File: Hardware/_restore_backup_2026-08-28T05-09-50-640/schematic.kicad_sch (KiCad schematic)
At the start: 6 parts, among them U1 ESP32-WROOM-32E, U2 HX711, U5 MAX30102, U6 MPU-6050

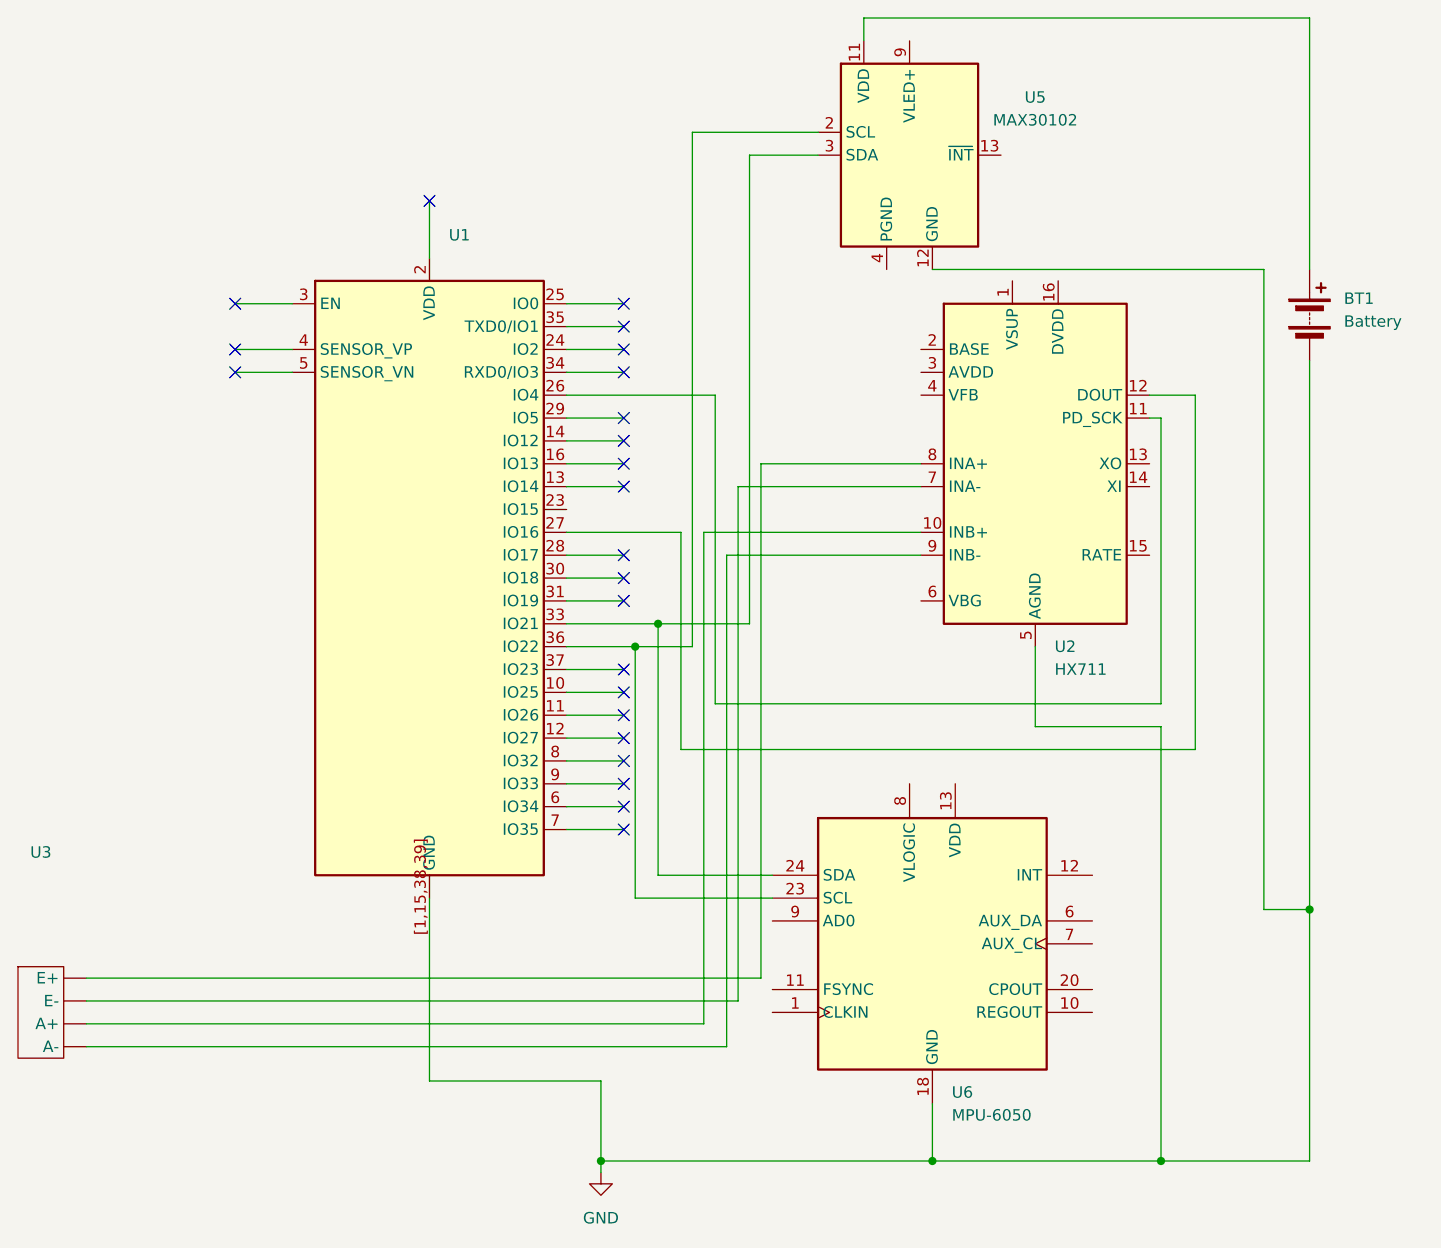
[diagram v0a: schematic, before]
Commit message: feat: added full structure to the project
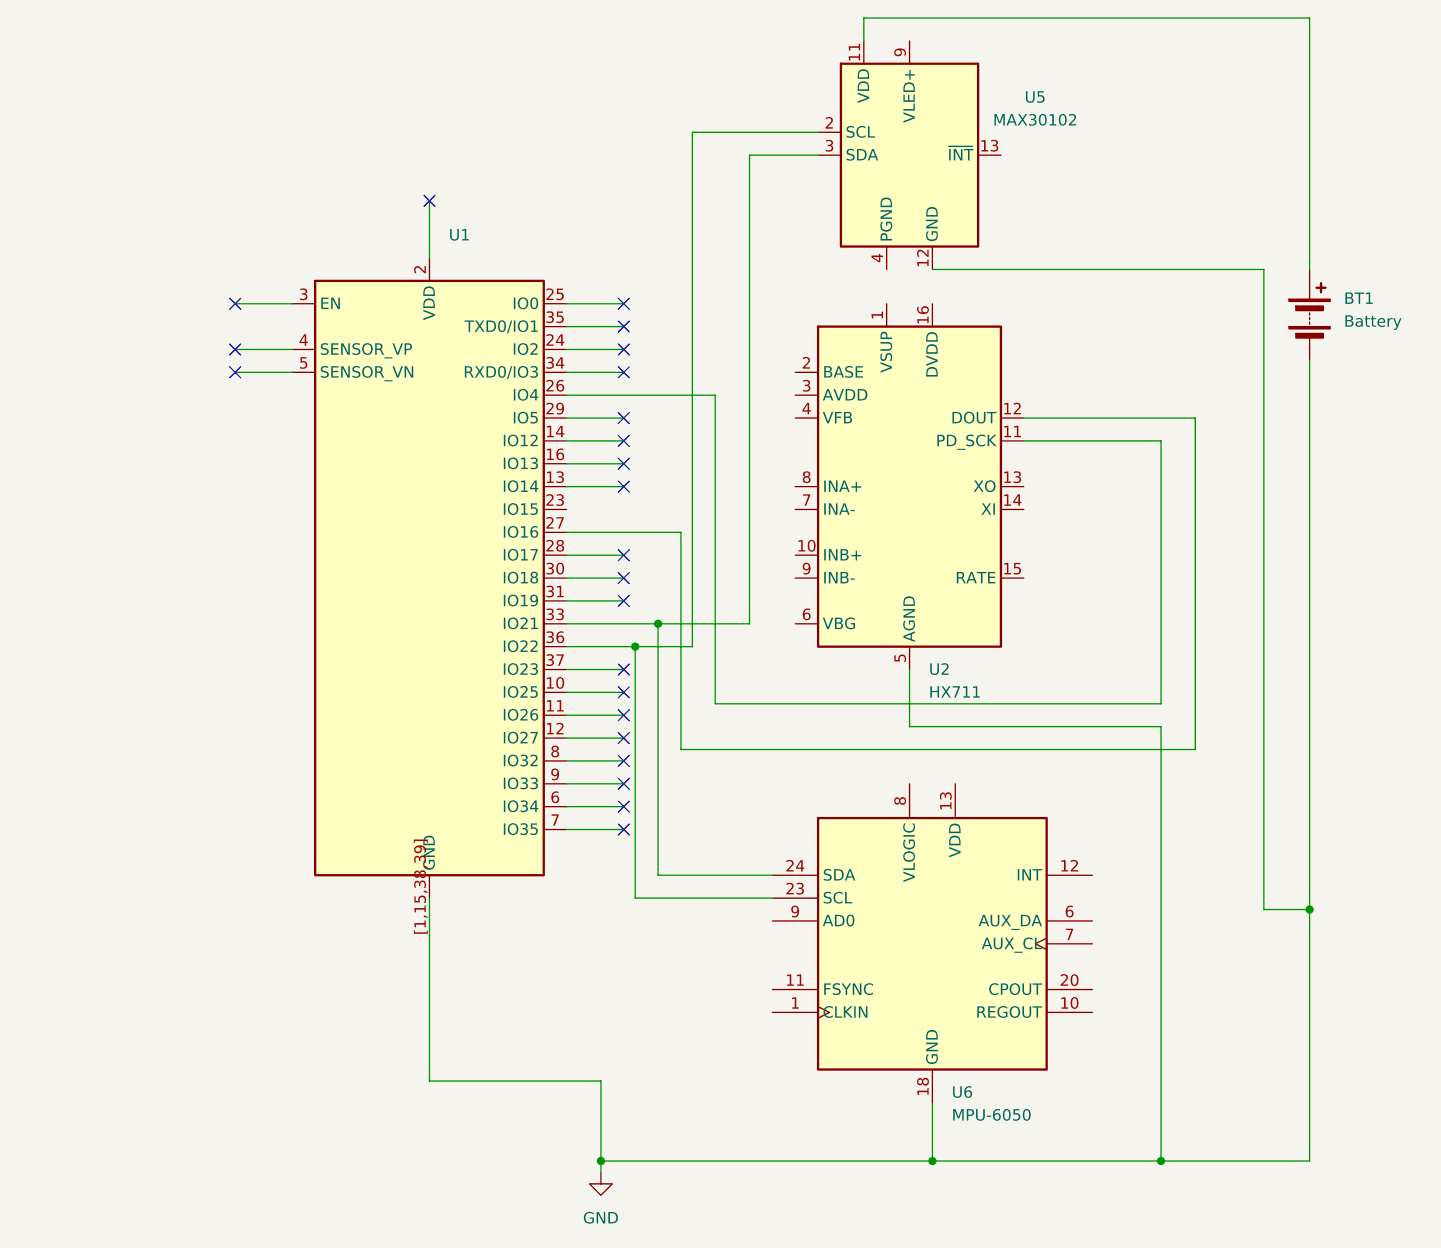
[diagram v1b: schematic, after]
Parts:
- removed U3: (no value), symbol New_Library:LOAD_CELL
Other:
- moved on the sheet: U2
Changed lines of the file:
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@@
-	(wire
-		(pts
-			(xy 179.07 78.74) (xy 196.85 78.74)
-		)
-		(stroke
-			(width 0)
-			(type default)
-		)
-	)
 	(wire
 		(pts
@@
 	(wire
 		(pts
-			(xy 172.72 86.36) (xy 196.85 86.36)
-		)
-		(stroke
-			(width 0)
-			(type default)
-		)
-	)
-	(wire
-		(pts
 			(xy 120.65 68.58) (xy 127 68.58)
 		)
@@
 	(wire
 		(pts
-			(xy 222.25 71.12) (xy 227.33 71.12)
-		)
-		(stroke
-			(width 0)
-			(type default)
-		)
-	)
-	(wire
-		(pts
-			(xy 176.53 138.43) (xy 176.53 81.28)
+			(xy 208.28 73.66) (xy 227.33 73.66)
 		)
 		(stroke
@@
 	(wire
 		(pts
-			(xy 104.14 140.97) (xy 172.72 140.97)
-		)
-		(stroke
-			(width 0)
-			(type default)
-		)
-	)
-	(wire
-		(pts
 			(xy 171.45 41.91) (xy 185.42 41.91)
 		)
@@
 	(wire
 		(pts
-			(xy 209.55 107.95) (xy 209.55 99.06)
+			(xy 195.58 107.95) (xy 195.58 101.6)
 		)
 		(stroke
@@
 	(wire
 		(pts
-			(xy 223.52 107.95) (xy 209.55 107.95)
+			(xy 223.52 107.95) (xy 195.58 107.95)
 		)
 		(stroke
@@
 	(wire
 		(pts
-			(xy 104.14 138.43) (xy 176.53 138.43)
-		)
-		(stroke
-			(width 0)
-			(type default)
-		)
-	)
-	(wire
-		(pts
 			(xy 163.83 101.6) (xy 157.48 101.6)
 		)
@@
 	(wire
 		(pts
-			(xy 172.72 140.97) (xy 172.72 86.36)
-		)
-		(stroke
-			(width 0)
-			(type default)
-		)
-	)
-	(wire
-		(pts
 			(xy 163.83 60.96) (xy 157.48 60.96)
 		)
@@
 	(wire
 		(pts
-			(xy 179.07 135.89) (xy 179.07 78.74)
-		)
-		(stroke
-			(width 0)
-			(type default)
-		)
-	)
-	(wire
-		(pts
 			(xy 142.24 147.32) (xy 161.29 147.32)
 		)
@@
 	(wire
 		(pts
-			(xy 176.53 81.28) (xy 196.85 81.28)
-		)
-		(stroke
-			(width 0)
-			(type default)
-		)
-	)
-	(wire
-		(pts
 			(xy 170.18 86.36) (xy 157.48 86.36)
 		)
@@
 	(wire
 		(pts
-			(xy 104.14 143.51) (xy 175.26 143.51)
-		)
-		(stroke
-			(width 0)
-			(type default)
-		)
-	)
-	(wire
-		(pts
 			(xy 163.83 68.58) (xy 157.48 68.58)
 		)
@@
 	(wire
 		(pts
-			(xy 175.26 88.9) (xy 196.85 88.9)
-		)
-		(stroke
-			(width 0)
-			(type default)
-		)
-	)
-	(wire
-		(pts
-			(xy 227.33 71.12) (xy 227.33 110.49)
-		)
-		(stroke
-			(width 0)
-			(type default)
-		)
-	)
-	(wire
-		(pts
-			(xy 223.52 73.66) (xy 223.52 105.41)
+			(xy 227.33 73.66) (xy 227.33 110.49)
+		)
+		(stroke
+			(width 0)
+			(type default)
+		)
+	)
+	(wire
+		(pts
+			(xy 223.52 76.2) (xy 223.52 105.41)
 		)
 		(stroke
@@
 	(wire
 		(pts
-			(xy 104.14 135.89) (xy 179.07 135.89)
-		)
-		(stroke
-			(width 0)
-			(type default)
-		)
-	)
-	(wire
-		(pts
 			(xy 223.52 105.41) (xy 173.99 105.41)
 		)
@@
 	(wire
 		(pts
-			(xy 175.26 143.51) (xy 175.26 88.9)
-		)
-		(stroke
-			(width 0)
-			(type default)
-		)
-	)
-	(wire
-		(pts
 			(xy 198.12 156.21) (xy 198.12 149.86)
 		)
@@
 	(wire
 		(pts
-			(xy 222.25 73.66) (xy 223.52 73.66)
+			(xy 208.28 76.2) (xy 223.52 76.2)
 		)
 		(stroke
@@
 	)
 	(symbol
-		(lib_id "New_Library:LOAD_CELL")
-		(at 100.33 124.46 0)
-		(unit 1)
-		(body_style 1)
-		(exclude_from_sim no)
-		(in_bom yes)
-		(on_board yes)
-		(in_pos_files yes)
-		(dnp no)
-		(fields_autoplaced yes)
-		(property "Reference" "U3"
-			(at 99.06 121.92 0)
-			(show_name no)
-			(do_not_autoplace no)
-			(effects
-				(font
-					(size 1.27 1.27)
-				)
-			)
-		)
-		(property "Value" ""
-			(at 100.33 124.46 0)
-			(show_name no)
-			(do_not_autoplace no)
-			(effects
-				(font
-					(size 1.27 1.27)
-				)
-			)
-		)
-		(property "Footprint" ""
-			(at 100.33 124.46 0)
-			(hide yes)
-			(show_name no)
-			(do_not_autoplace no)
-			(effects
-				(font
-					(size 1.27 1.27)
-				)
-			)
-		)
-		(property "Datasheet" ""
-			(at 100.33 124.46 0)
-			(hide yes)
-			(show_name no)
-			(do_not_autoplace no)
-			(effects
-				(font
-					(size 1.27 1.27)
-				)
-			)
-		)
-		(property "Description" ""
-			(at 100.33 124.46 0)
-			(hide yes)
-			(show_name no)
-			(do_not_autoplace no)
-			(effects
-				(font
-					(size 1.27 1.27)
-				)
-			)
-		)
-		(pin ""
-		)
-		(pin ""
-		)
-		(pin ""
-		)
-		(pin ""
-		)
-		(instances
-			(project "schematic"
-				(path "/62d25dba-bbf5-4c29-afa2-e2397d4820c7"
-					(reference "U3")
-					(unit 1)
-				)
-			)
-		)
-	)
-	(symbol
 		(lib_id "Analog_ADC:HX711")
-		(at 209.55 78.74 0)
+		(at 195.58 81.28 0)
 		(unit 1)
 		(body_style 1)
@@
 		(fields_autoplaced yes)
 		(property "Reference" "U2"
-			(at 211.6933 99.06 0)
+			(at 197.7233 101.6 0)
 			(show_name no)
 			(do_not_autoplace no)
@@
 		)
 		(property "Value" "HX711"
-			(at 211.6933 101.6 0)
+			(at 197.7233 104.14 0)
 			(show_name no)
 			(do_not_autoplace no)
@@
 		)
 		(property "Footprint" "Package_SO:SOIC-16_3.9x9.9mm_P1.27mm"
-			(at 213.36 77.47 0)
+			(at 199.39 80.01 0)
 			(hide yes)
 			(show_name no)
@@
 		)
 		(property "Datasheet" "https://web.archive.org/web/20220615044707/https://akizukidenshi.com/download/ds/avia/hx711.pdf"
-			(at 213.36 80.01 0)
+			(at 199.39 82.55 0)
 			(hide yes)
 			(show_name no)
@@
 		)
 		(property "Description" "24-bit Analog-to-Digital Converter (ADC) for Weight Scales, SOIC-16 (SOP-16)"
-			(at 209.55 78.74 0)
-			(hide yes)
-			(show_name no)
+			(at 195.58 81.28 0)
+			(hide yes)
+			(show_name no)
